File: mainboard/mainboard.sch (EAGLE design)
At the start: 30 parts, among them IC1 ATMEGA168-PU

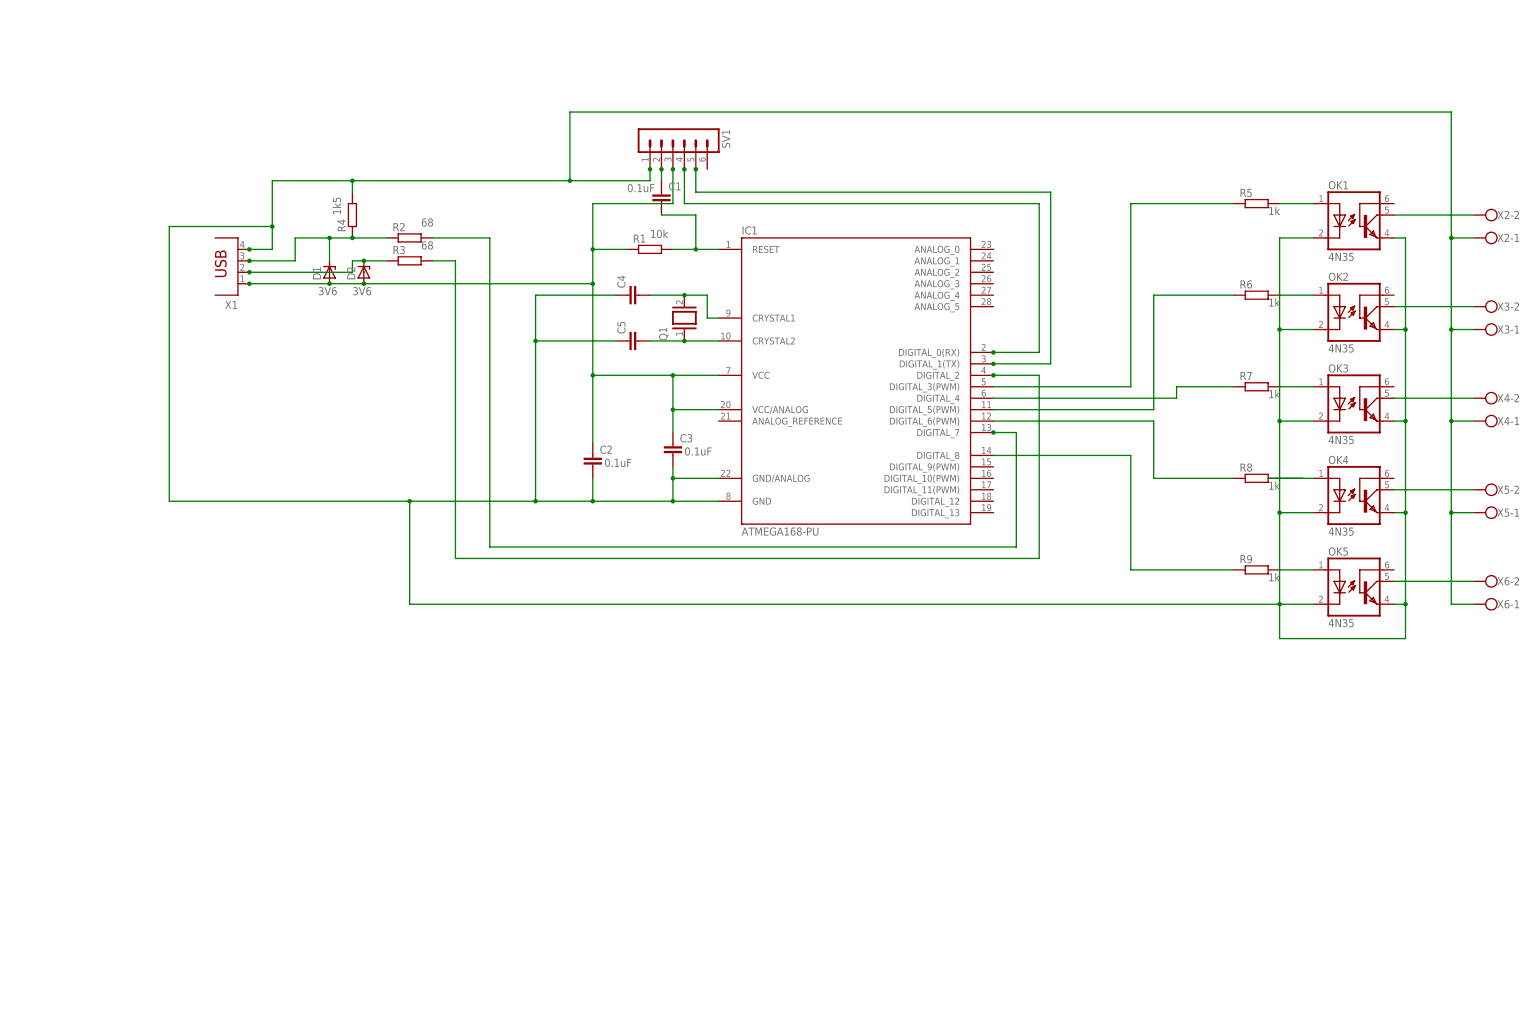
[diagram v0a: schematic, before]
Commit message: added thermocouple interface chips and terminals
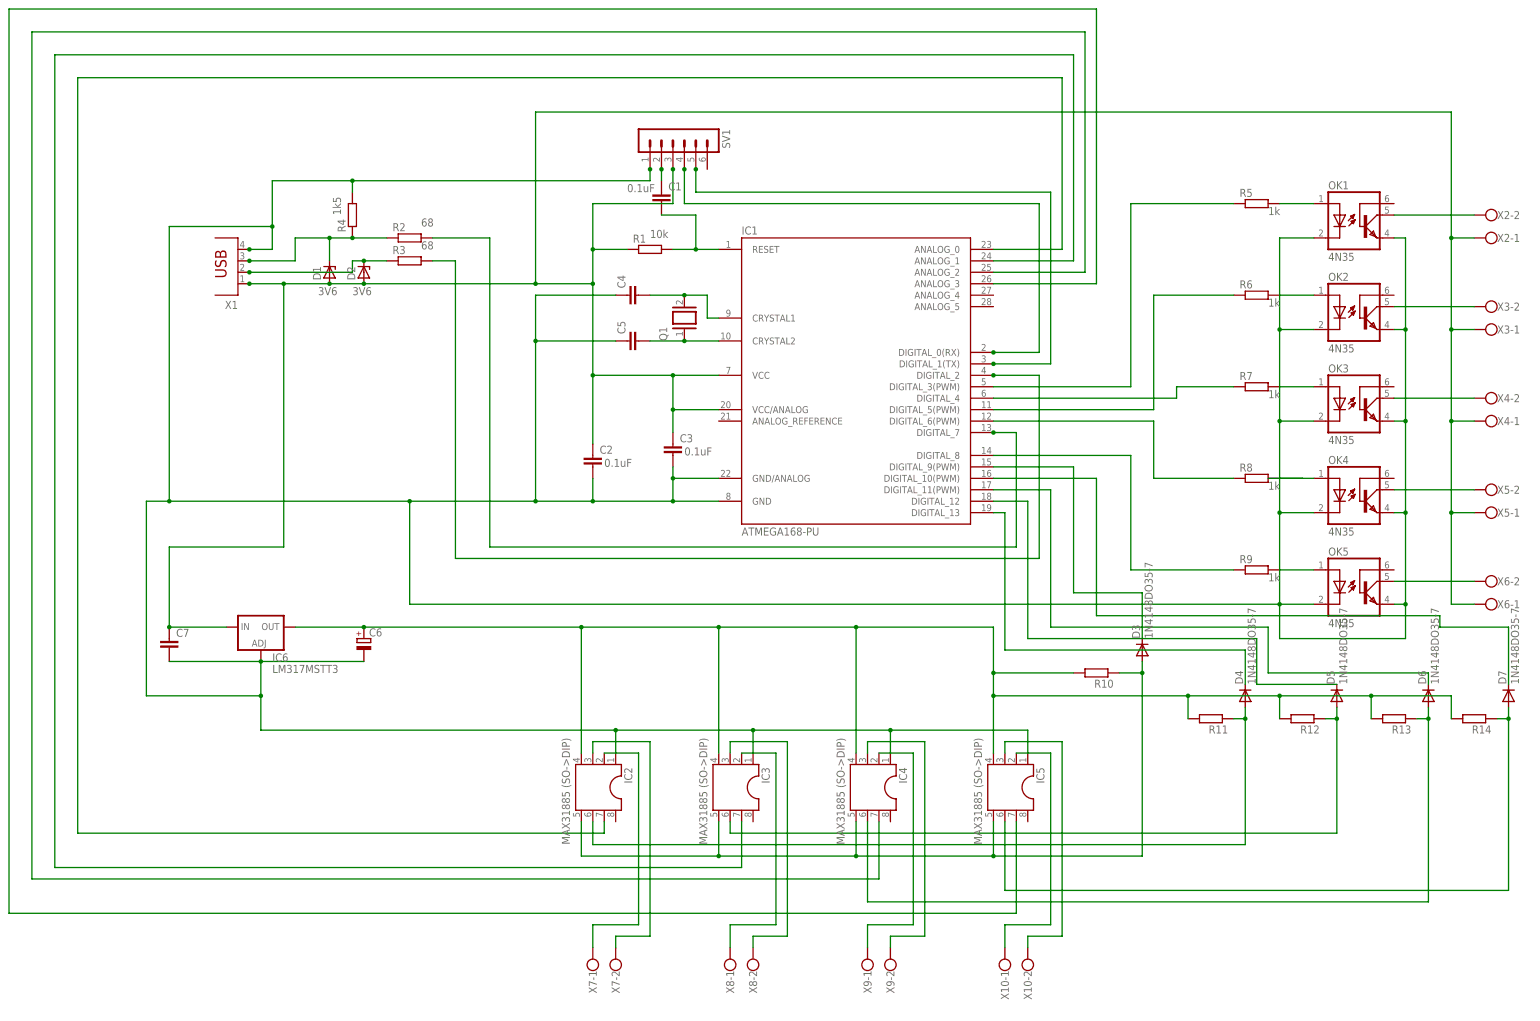
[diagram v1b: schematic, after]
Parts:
- added C6: (no value), resistor:CPOL-EU153CLV-0605
- added C7: (no value), capacitor-wima:C2,5-3
- added D3, D4, D5, D6, D7: 1N4148DO35-7, diode:1N4148DO35-7
- added IC2, IC3, IC4, IC5: (no value), ic-package:DIL8S
- added IC6: LM317MSTT3, v-reg-mod:LM317MSTT3
- added R10, R11, R12, R13, R14: (no value), resistor:R-EU_0204/7
- added X10, X7, X8, X9: (no value), con-wago-500:W237-102
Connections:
- new net N$28: IC2.2, X7-1.KL
- new net N$29: C2.2, C3.2, C4.1, C5.1, C6.-, C7.2, IC1.GND, IC1.GND/ANALOG, IC2.1, IC3.1, IC4.1, IC5.1, IC6.ADJ, OK1.C, OK1.EMI, OK2.C, OK2.EMI, OK3.C, OK3.EMI, OK4.C, OK4.EMI, OK5.C, OK5.EMI, R4.2, SV1.1, X1.4
- new net N$30: C6.+, IC2.4, IC3.4, IC4.4, IC5.4, IC6.OUT, R10.2, R11.2, R12.2, R13.2, R14.2
- new net N$31: IC3.3, X8-2.KL
- new net N$32: IC4.3, X9-2.KL
- new net N$33: IC5.3, X10-2.KL
- new net N$34: IC3.2, X8-1.KL
- new net N$35: IC4.2, X9-1.KL
- new net N$36: IC5.2, X10-1.KL
- new net N$37: D3.A, IC2.5, IC3.5, IC4.5, IC5.5, R10.1
- new net N$38: D3.C, IC1.DIGITAL_9(PWM)
- new net N$39: D5.A, IC3.6, R12.1
- new net N$40: D4.A, IC2.6, R11.1
- new net N$41: D6.A, IC4.6, R13.1
- new net N$42: D7.A, IC5.6, R14.1
- new net N$43: D4.C, IC1.DIGITAL_13
- new net N$44: D5.C, IC1.DIGITAL_12
- new net N$45: D6.C, IC1.DIGITAL_11(PWM)
- new net N$46: D7.C, IC1.DIGITAL_10(PWM)
- new net N$47: IC1.ANALOG_0, IC2.7
- new net N$48: IC1.ANALOG_1, IC3.7
- new net N$49: IC1.ANALOG_2, IC4.7
- new net N$50: IC1.ANALOG_3, IC5.7
- net N$3: now also C7.1, IC6.IN, X2-1.KL, X3-1.KL, X4-1.KL, X5-1.KL, X6-1.KL
- net N$9: now also IC2.3, X7-2.KL; no longer C2.2, C3.2, C4.1, C5.1, IC1.GND, IC1.GND/ANALOG, OK1.C, OK1.EMI, OK2.C, OK2.EMI, OK3.C, OK3.EMI, OK4.C, OK4.EMI, OK5.C, OK5.EMI, R4.2, SV1.1, X1.4, X2-1.KL, X3-1.KL, X4-1.KL, X5-1.KL, X6-1.KL
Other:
- note added: "MAX31885 (SO->DIP)"
